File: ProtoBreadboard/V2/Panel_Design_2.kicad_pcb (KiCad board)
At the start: 2 copper layers, 126.5 x 65.5 mm, 24 parts, among them IC1 AT90USB1286-AU, J1 Conn_01x30_Female, J11 Conn_01x32_Female, J12 Conn_01x06_Female, J19 Conn_01x02_Female, J23 Conn_01x02_Female, J3 Conn_01x32_Female, J5 Conn_01x30_Female, J8 Conn_01x06_Female, SW1 RotaryEncoder_Switch, SW2 RotaryEncoder_Switch, U1 IS31FL3741A, U3 PRTR5V0U2X

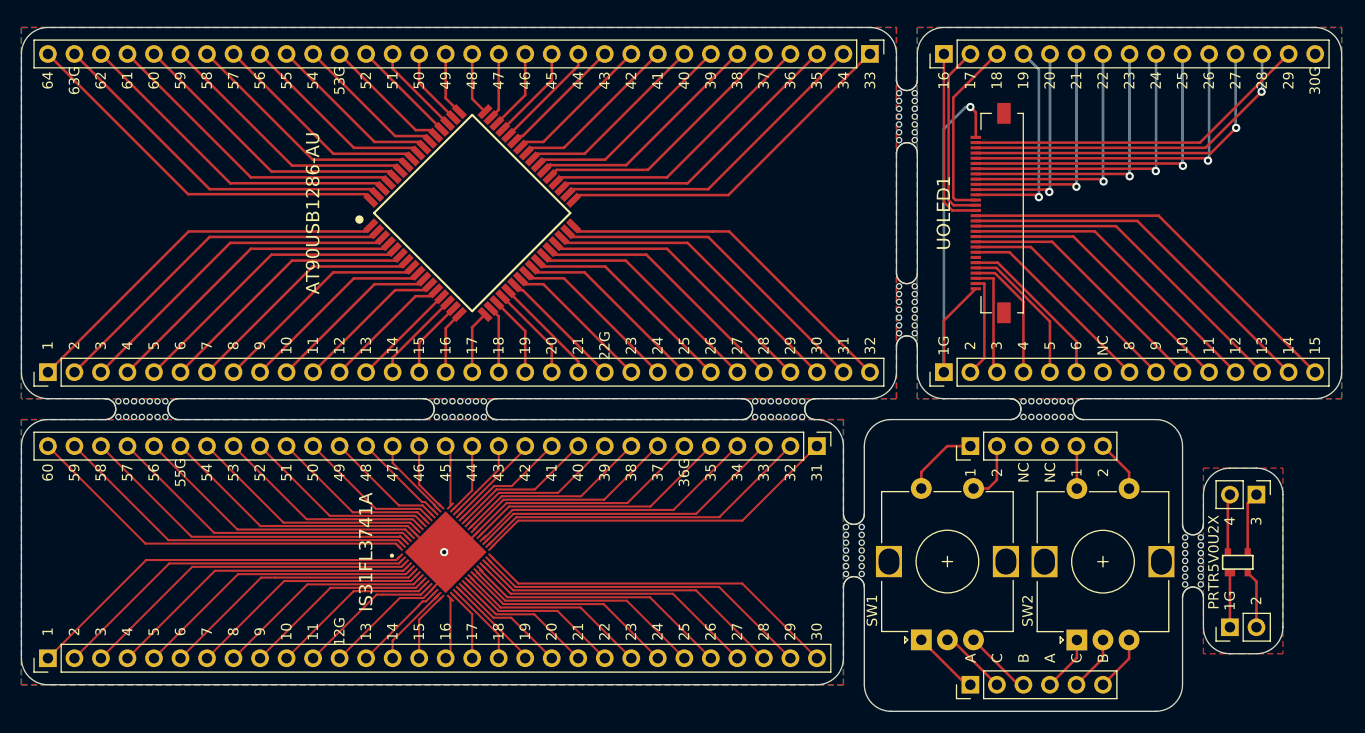
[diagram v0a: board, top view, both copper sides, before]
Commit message: Added Gerber Files for all 3 new designs
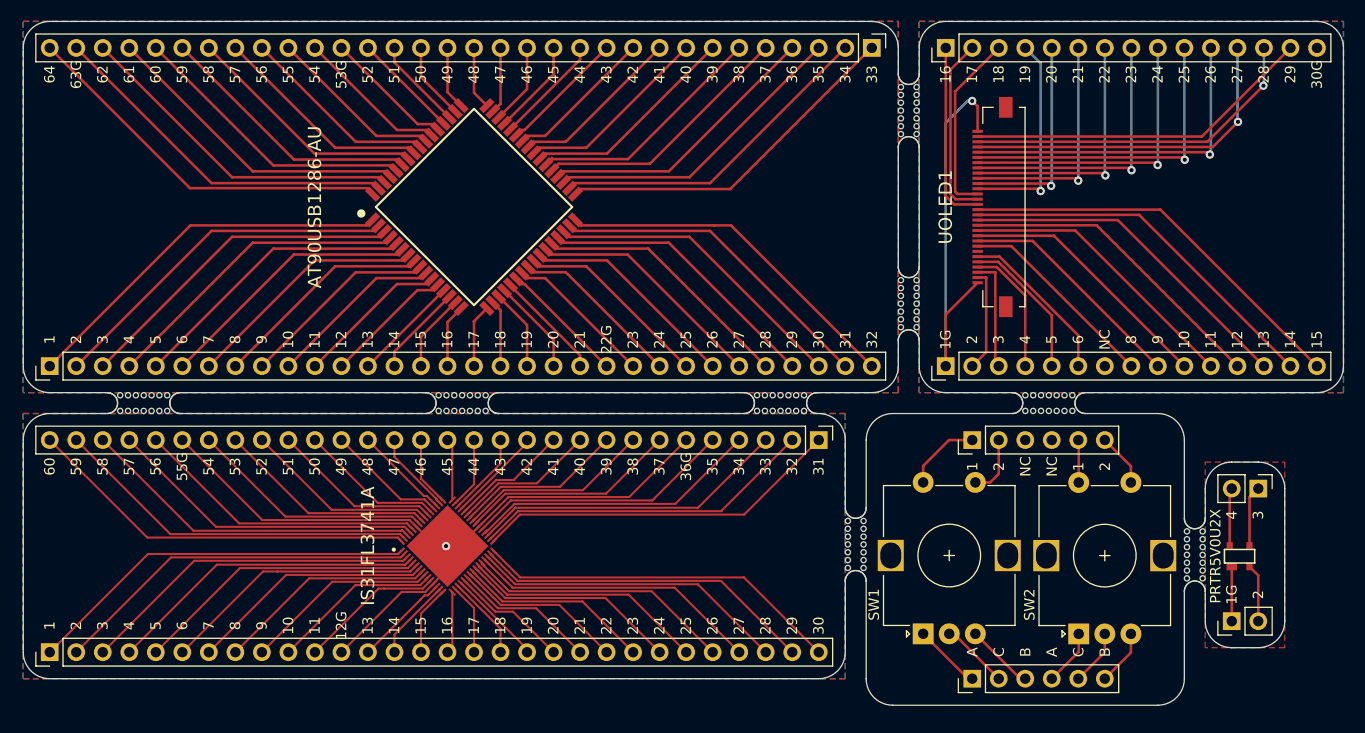
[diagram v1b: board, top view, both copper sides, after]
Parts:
- moved J19 0.61 mm to (141.7, 77.8)
- moved J1 0.61 mm to (28.5, 80.7)
- moved SW2 0.61 mm to (127.1, 79.0)
- moved J23 0.61 mm to (144.3, 65.1)
- moved IC1 0.61 mm to (69.1, 38.1)
- moved J11 0.61 mm to (107.2, 22.9)
- moved J12 0.61 mm to (116.9, 60.4)
- moved J3 0.61 mm to (28.5, 53.3)
- moved J5 0.61 mm to (102.2, 60.4)
- moved JOLED2 0.61 mm to (114.3, 22.9)
- moved UOLED1 0.61 mm to (119.4, 38.1)
- moved mouse-bite-2mm-slot 0.61 mm to (98.5, 56.9)
- moved mouse-bite-2mm-slot 0.61 mm to (110.8, 47.4)
- moved mouse-bite-2mm-slot 0.61 mm to (124.2, 56.9)
- moved mouse-bite-2mm-slot 0.61 mm to (110.8, 28.9)
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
